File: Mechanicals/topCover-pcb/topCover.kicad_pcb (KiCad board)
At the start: 2 copper layers, 89 x 100 mm, 1 part

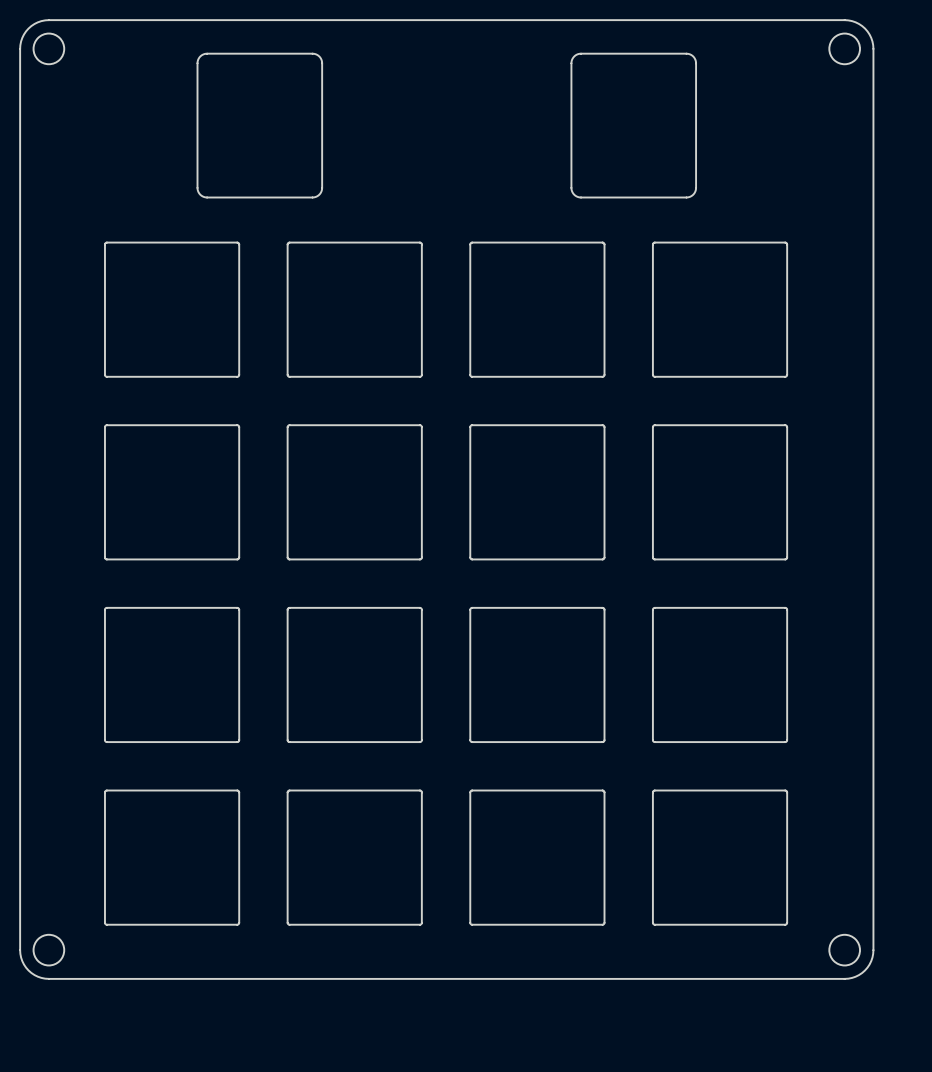
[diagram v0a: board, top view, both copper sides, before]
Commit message: update board
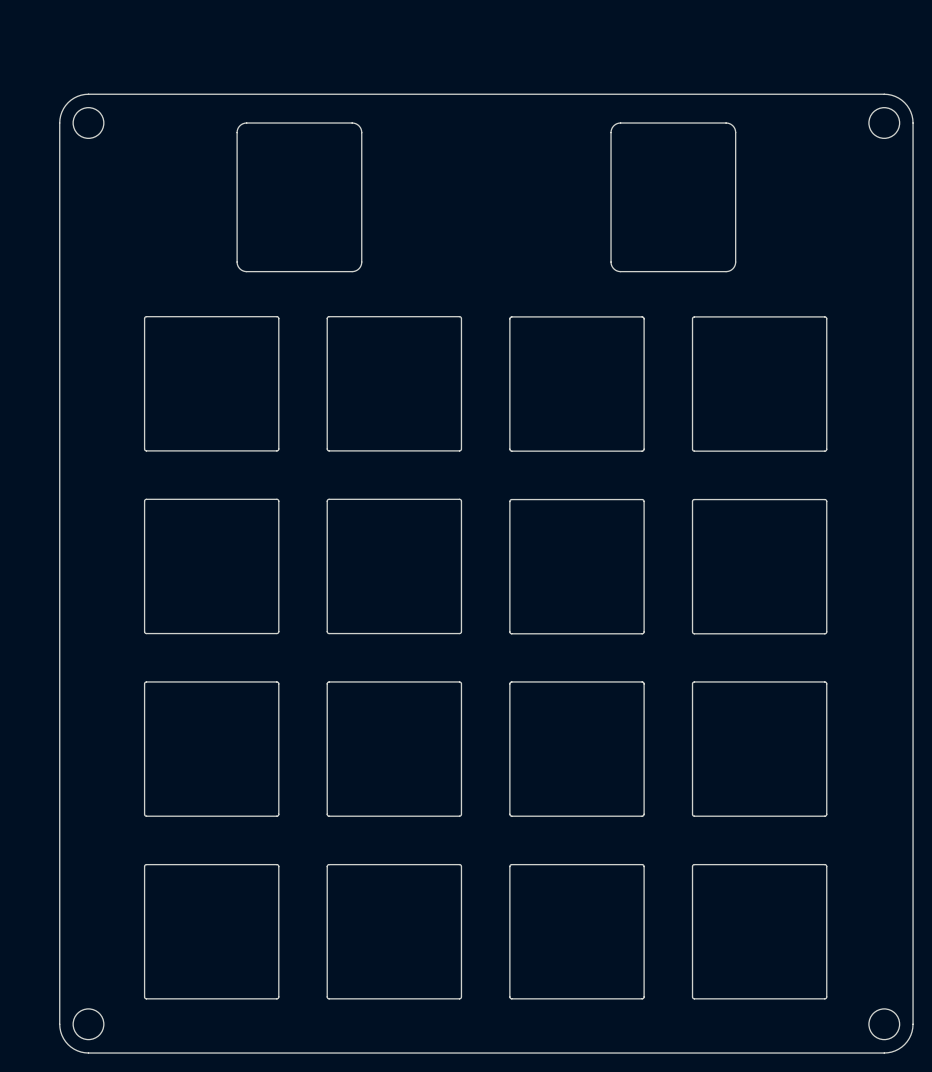
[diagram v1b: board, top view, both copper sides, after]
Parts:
- removed the REF** at (143.9, 98.6)
- added REF**: MountingHole_3.2mm_M3, MountingHole:MountingHole_3.2mm_M3, F.Cu at (188.2, 148.6)
- added REF**: MountingHole_3.2mm_M3, MountingHole:MountingHole_3.2mm_M3, F.Cu at (105.2, 148.6)
- added REF**: MountingHole_3.2mm_M3, MountingHole:MountingHole_3.2mm_M3, F.Cu at (105.2, 54.5)
- added REF**: MountingHole_3.2mm_M3, MountingHole:MountingHole_3.2mm_M3, F.Cu at (188.2, 54.5)
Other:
- outline, holes or cut-outs redrawn
